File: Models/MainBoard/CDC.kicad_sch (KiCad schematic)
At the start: 5 parts, among them U7 AD7745

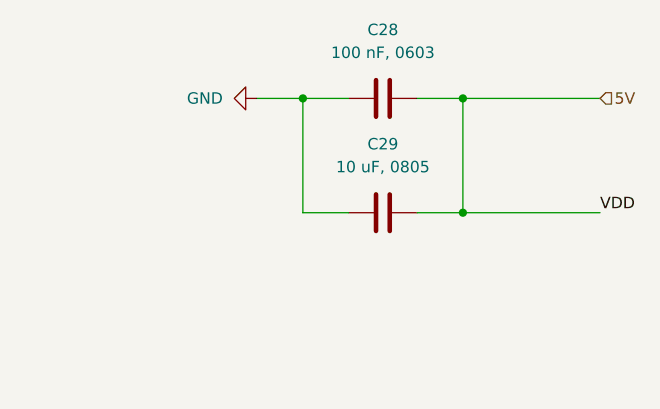
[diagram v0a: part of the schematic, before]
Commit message: Save progress
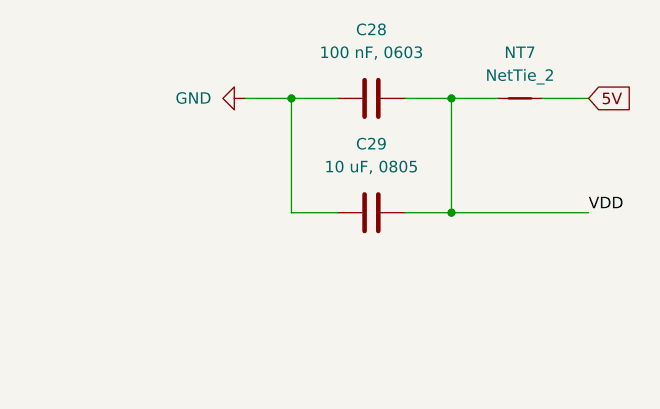
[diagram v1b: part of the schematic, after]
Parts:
- added NT7: NetTie_2, symbol Device:NetTie_2
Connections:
- net 5V: now also NT7.2; no longer C28.2, C29.2, R8.1, R9.1, U7.14 (VDD)
- new net VDD: C28.2, C29.2, NT7.1, R8.1, R9.1, U7.14 (VDD)
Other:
- moved on the sheet: C28, C29
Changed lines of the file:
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@@
 	(paper "A4")
-	(junction
-		(at 227.33 50.8)
-		(diameter 0)
-		(color 0 0 0 0)
-	)
 	(junction
 		(at 132.08 78.74)
@@
 	)
 	(junction
+		(at 226.06 50.8)
+		(diameter 0)
+		(color 0 0 0 0)
+	)
+	(junction
 		(at 91.44 78.74)
 		(diameter 0)
@@
 	)
 	(junction
-		(at 227.33 63.5)
+		(at 226.06 63.5)
 		(diameter 0)
 		(color 0 0 0 0)
 	)
 	(junction
-		(at 209.55 50.8)
+		(at 208.28 50.8)
 		(diameter 0)
 		(color 0 0 0 0)
@@
 	(wire
 		(pts
-			(xy 204.47 50.8) (xy 209.55 50.8)
+			(xy 236.22 50.8) (xy 241.3 50.8)
+		)
+		(stroke
+			(width 0)
+			(type default)
+		)
+	)
+	(wire
+		(pts
+			(xy 203.2 50.8) (xy 208.28 50.8)
 		)
 		(stroke
@@
 	(wire
 		(pts
-			(xy 222.25 63.5) (xy 227.33 63.5)
+			(xy 220.98 63.5) (xy 226.06 63.5)
 		)
 		(stroke
@@
 	(wire
 		(pts
-			(xy 209.55 63.5) (xy 214.63 63.5)
+			(xy 208.28 63.5) (xy 213.36 63.5)
 		)
 		(stroke
@@
 	(wire
 		(pts
-			(xy 214.63 50.8) (xy 209.55 50.8)
+			(xy 213.36 50.8) (xy 208.28 50.8)
 		)
 		(stroke
@@
 	(wire
 		(pts
-			(xy 222.25 50.8) (xy 227.33 50.8)
+			(xy 220.98 50.8) (xy 226.06 50.8)
 		)
 		(stroke
@@
 	(wire
 		(pts
+			(xy 226.06 50.8) (xy 231.14 50.8)
+		)
+		(stroke
+			(width 0)
+			(type default)
+		)
+	)
+	(wire
+		(pts
 			(xy 96.52 83.82) (xy 99.06 83.82)
 		)
@@
 	(wire
 		(pts
-			(xy 227.33 63.5) (xy 242.57 63.5)
+			(xy 226.06 63.5) (xy 241.3 63.5)
 		)
 		(stroke
@@
 	(wire
 		(pts
-			(xy 227.33 50.8) (xy 242.57 50.8)
-		)
-		(stroke
-			(width 0)
-			(type default)
-		)
-	)
-	(wire
-		(pts
 			(xy 96.52 96.52) (xy 99.06 96.52)
 		)
@@
 	(wire
 		(pts
-			(xy 227.33 63.5) (xy 227.33 50.8)
-		)
-		(stroke
-			(width 0)
-			(type default)
-		)
-	)
-	(wire
-		(pts
-			(xy 209.55 50.8) (xy 209.55 63.5)
+			(xy 226.06 63.5) (xy 226.06 50.8)
+		)
+		(stroke
+			(width 0)
+			(type default)
+		)
+	)
+	(wire
+		(pts
+			(xy 208.28 50.8) (xy 208.28 63.5)
 		)
 		(stroke
@@
 	)
 	(label "VDD"
-		(at 242.57 63.5 0)
+		(at 241.3 63.5 0)
 		(effects
 			(font
@@
 		)
 	)
-	(hierarchical_label "5V"
+	(global_label "5V"
 		(shape input)
-		(at 242.57 50.8 0)
+		(at 241.3 50.8 0)
+		(fields_autoplaced yes)
 		(effects
 			(font
@@
 			)
 			(justify left)
+		)
+		(property "Intersheetrefs" "${INTERSHEET_REFS}"
+			(at 246.5833 50.8 0)
+			(effects
+				(font
+					(size 1.27 1.27)
+				)
+				(justify left)
+				(hide yes)
+			)
 		)
 	)
@@
 	(symbol
 		(lib_id "power:GND")
-		(at 204.47 50.8 270)
+		(at 203.2 50.8 270)
 		(unit 1)
 		(exclude_from_sim no)
@@
 		(fields_autoplaced yes)
 		(property "Reference" "#PWR026"
-			(at 198.12 50.8 0)
+			(at 196.85 50.8 0)
 			(effects
 				(font
@@
 		)
 		(property "Value" "GND"
-			(at 200.66 50.7999 90)
+			(at 199.39 50.7999 90)
 			(effects
 				(font
@@
 		)
 		(property "Footprint" ""
-			(at 204.47 50.8 0)
+			(at 203.2 50.8 0)
 			(effects
 				(font
@@
 		)
 		(property "Datasheet" ""
-			(at 204.47 50.8 0)
+			(at 203.2 50.8 0)
 			(effects
 				(font
@@
 		)
 		(property "Description" "Power symbol creates a global label with name \"GND\" , ground"
-			(at 204.47 50.8 0)
+			(at 203.2 50.8 0)
 			(effects
 				(font
@@
 	(symbol
 		(lib_id "Device:C")
-		(at 218.44 50.8 90)
+		(at 217.17 50.8 90)
 		(unit 1)
 		(exclude_from_sim no)
@@
 		(fields_autoplaced yes)
 		(property "Reference" "C28"
-			(at 218.44 43.18 90)
+			(at 217.17 43.18 90)
 			(effects
 				(font
@@
 		)
 		(property "Value" "100 nF, 0603"
-			(at 218.44 45.72 90)
+			(at 217.17 45.72 90)
 			(effects
 				(font
@@
 		)
 		(property "Footprint" ""
-			(at 222.25 49.8348 0)
+			(at 220.98 49.8348 0)
 			(effects
 				(font
@@
 		)
 		(property "Datasheet" "~"
-			(at 218.44 50.8 0)
+			(at 217.17 50.8 0)
 			(effects
 				(font
@@
 		)
 		(property "Description" "Unpolarized capacitor"
-			(at 218.44 50.8 0)
+			(at 217.17 50.8 0)
 			(effects
 				(font
@@
 		)
 		(property "Purchase Link" ""
-			(at 218.44 50.8 0)
+			(at 217.17 50.8 0)
 			(effects
 				(font
@@
 	)
 	(symbol
+		(lib_id "Device:NetTie_2")
+		(at 233.68 50.8 0)
+		(unit 1)
+		(exclude_from_sim no)
+		(in_bom no)
+		(on_board yes)
+		(dnp no)
+		(fields_autoplaced yes)
+		(property "Reference" "NT7"
+			(at 233.68 45.72 0)
+			(effects
+				(font
+					(size 1.27 1.27)
+				)
+			)
+		)
+		(property "Value" "NetTie_2"
+			(at 233.68 48.26 0)
+			(effects
+				(font
+					(size 1.27 1.27)
+				)
+			)
+		)
+		(property "Footprint" ""
+			(at 233.68 50.8 0)
+			(effects
+				(font
+					(size 1.27 1.27)
+				)
+				(hide yes)
+			)
+		)
+		(property "Datasheet" "~"
+			(at 233.68 50.8 0)
+			(effects
+				(font
+					(size 1.27 1.27)
+				)
+				(hide yes)
+			)
+		)
+		(property "Description" "Net tie, 2 pins"
+			(at 233.68 50.8 0)
+			(effects
+				(font
+					(size 1.27 1.27)
+				)
+				(hide yes)
+			)
+		)
+		(pin "1"
+		)
+		(pin "2"
+		)
+		(instances
+			(project ""
+				(path "/600cc1cc-74ca-4bfc-97a0-b230eb3afbcd/812a2394-e6f7-4194-9eea-57be5665ec29"
+					(reference "NT7")
+					(unit 1)
+				)
+			)
+		)
+	)
+	(symbol
 		(lib_id "Device:C")
-		(at 218.44 63.5 90)
+		(at 217.17 63.5 90)
 		(unit 1)
 		(exclude_from_sim no)
@@
 		(fields_autoplaced yes)
 		(property "Reference" "C29"
-			(at 218.44 55.88 90)
+			(at 217.17 55.88 90)
 			(effects
 				(font
@@
 		)
 		(property "Value" "10 uF, 0805"
-			(at 218.44 58.42 90)
+			(at 217.17 58.42 90)
 			(effects
 				(font
@@
 		)
 		(property "Footprint" ""
-			(at 222.25 62.5348 0)
+			(at 220.98 62.5348 0)
 			(effects
 				(font
@@
 		)
 		(property "Datasheet" "~"
-			(at 218.44 63.5 0)
+			(at 217.17 63.5 0)
 			(effects
 				(font
@@
 		)
 		(property "Description" "Unpolarized capacitor"
-			(at 218.44 63.5 0)
+			(at 217.17 63.5 0)
 			(effects
 				(font
@@
 		)
 		(property "Purchase Link" ""
-			(at 218.44 63.5 0)
-			(effects
-				(font
+			(at 217.17 63.5 0)
+			(effects
+				(font
